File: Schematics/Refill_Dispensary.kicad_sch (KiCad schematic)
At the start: 60 parts, among them J1 USB_B_Micro, J10 Switch 2, J11 Switch 3, J12 Switch 1, J2 Pot 1, J3 Barrel_Jack_Switch, J4 USB_BOOT, J5 Load Cell Power, J6 Load Cell Data, J7 Inductor 1, J8 Inductor 2, J9 Pot 2, Q1 TIP120, Q2 TIP120, SW4 SW_SPDT, U1 RP2040, U2 NCP1117-3.3_SOT223, U3 Flash Memory, U4 NHD-C0220BIZ, U5 AD622, Y1 Crystal

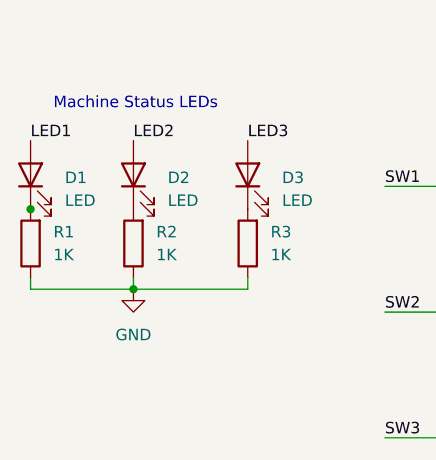
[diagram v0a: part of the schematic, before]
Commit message: changes
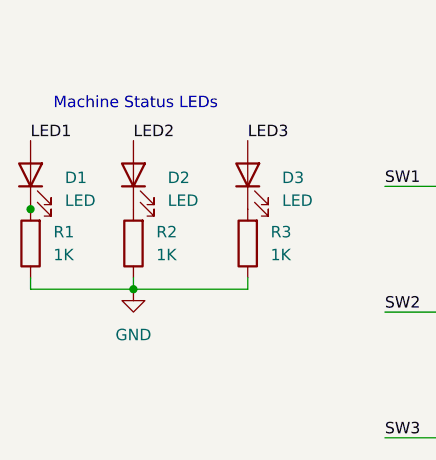
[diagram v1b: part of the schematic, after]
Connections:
- net GND: now also R1.1
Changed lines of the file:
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@@
-    (stroke (width 0) (type default) (color 0 0 0 0))
-  )
-  (wire (pts (xy 20.32 250.2159) (xy 20.32 251.46))
     (stroke (width 0) (type default) (color 0 0 0 0))
   )
@@
     (stroke (width 0) (type default) (color 0 0 0 0))
   )
+  (wire (pts (xy 20.32 250.19) (xy 20.32 251.46))
+    (stroke (width 0) (type default) (color 0 0 0 0))
+  )
